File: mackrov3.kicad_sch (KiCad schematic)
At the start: 31 parts, among them SW1 SW_Push, U1 ProMicro

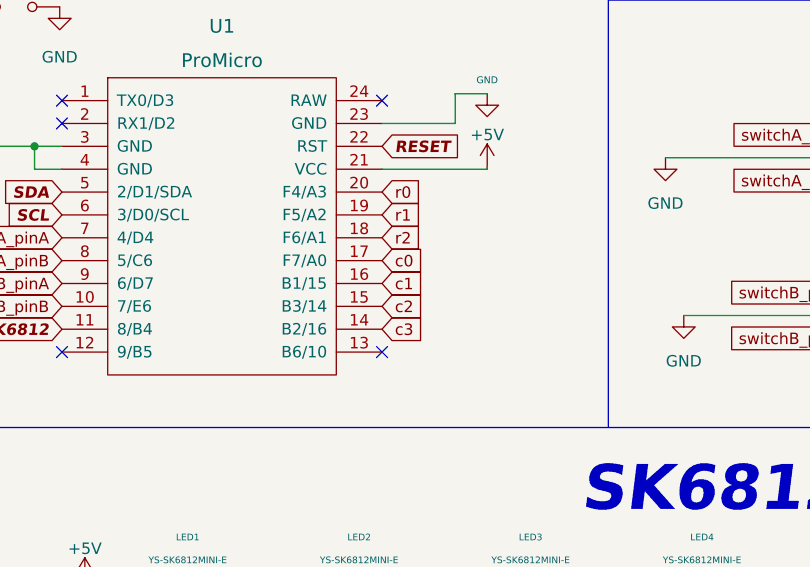
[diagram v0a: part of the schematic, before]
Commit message: Add updates
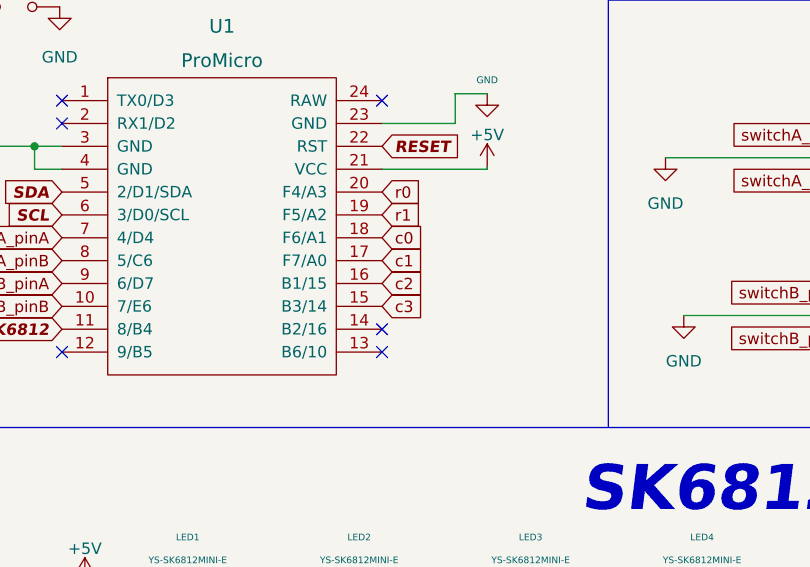
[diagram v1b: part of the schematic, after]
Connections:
- net r2 is gone; now on net c0: U1.18 (F6/A1)
- net c0: no longer U1.17 (F7/A0)
- net c1: now also U1.17 (F7/A0); no longer U1.16 (B1/15)
- net c2: now also U1.16 (B1/15); no longer U1.15 (B3/14)
- net c3: now also U1.15 (B3/14); no longer U1.14 (B2/16)
- no-connect marks 6 -> 7
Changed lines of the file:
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@@
   (junction (at 232.664 141.986) (diameter 0) (color 0 0 0 0)
   )
+  (no_connect (at 73.152 142.24))
   (no_connect (at 153.924 177.8))
   (no_connect (at 37.592 119.38))
@@
     )
   )
-  (global_label "c2" (shape input) (at 73.152 139.7 0) (fields_autoplaced)
-    (effects (font (size 1.27 1.27)) (justify left))
-    (property "Intersheet References" "${INTERSHEET_REFS}" (id 0) (at 99.822 -1.27 0)
+  (global_label "c2" (shape input) (at 73.152 137.16 0) (fields_autoplaced)
+    (effects (font (size 1.27 1.27)) (justify left))
+    (property "Intersheet References" "${INTERSHEET_REFS}" (id 0) (at 99.822 -3.81 0)
       (effects (font (size 1.27 1.27)) hide)
     )
@@
     )
   )
-  (global_label "r2" (shape input) (at 73.152 132.08 0) (fields_autoplaced)
-    (effects (font (size 1.27 1.27)) (justify left))
-    (property "Intersheet References" "${INTERSHEET_REFS}" (id 0) (at 77.5608 132.1594 0)
-      (effects (font (size 1.27 1.27)) (justify left) hide)
-    )
-  )
   (global_label "switchA_pinB" (shape input) (at 125.984 125.73 180) (fields_autoplaced)
     (effects (font (size 1.27 1.27)) (justify right))
@@
     )
   )
-  (global_label "c0" (shape input) (at 73.152 134.62 0) (fields_autoplaced)
-    (effects (font (size 1.27 1.27)) (justify left))
-    (property "Intersheet References" "${INTERSHEET_REFS}" (id 0) (at 99.822 19.05 0)
+  (global_label "c0" (shape input) (at 73.152 132.08 0) (fields_autoplaced)
+    (effects (font (size 1.27 1.27)) (justify left))
+    (property "Intersheet References" "${INTERSHEET_REFS}" (id 0) (at 99.822 16.51 0)
       (effects (font (size 1.27 1.27)) hide)
     )
@@
     )
   )
-  (global_label "c3" (shape input) (at 73.152 142.24 0) (fields_autoplaced)
-    (effects (font (size 1.27 1.27)) (justify left))
-    (property "Intersheet References" "${INTERSHEET_REFS}" (id 0) (at 77.8632 142.1606 0)
+  (global_label "c3" (shape input) (at 73.152 139.7 0) (fields_autoplaced)
+    (effects (font (size 1.27 1.27)) (justify left))
+    (property "Intersheet References" "${INTERSHEET_REFS}" (id 0) (at 77.8632 139.6206 0)
       (effects (font (size 1.27 1.27)) (justify left) hide)
     )
@@
     )
   )
-  (global_label "c1" (shape input) (at 73.152 137.16 0) (fields_autoplaced)
-    (effects (font (size 1.27 1.27)) (justify left))
-    (property "Intersheet References" "${INTERSHEET_REFS}" (id 0) (at 99.822 8.89 0)
-      (effects (font (size 1.27 1.27)) hide)
-    )
+  (global_label "c1" (shape input) (at 73.152 134.62 0) (fields_autoplaced)
+    (effects (font (size 1.27 1.27)) (justify left))
+    (property "Intersheet References" "${INTERSHEET_REFS}" (id 0) (at 99.822 6.35 0)
+      (effects (font (size 1.27 1.27)) hide)
+    )
